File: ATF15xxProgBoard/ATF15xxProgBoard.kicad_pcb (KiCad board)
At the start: 4 copper layers, 71.1 x 96.2 mm, 42 parts, among them J1 Conn_02x05_Odd_Even, J10 Conn_02x03_Odd_Even, J2 Conn_02x07_Odd_Even, J6 Conn_02x16_Counter_Clockwise, J7 Conn_02x16_Counter_Clockwise, J8 Conn_02x03_Odd_Even, J9 USB_C, U3 ATmega32U4-AU, U4 MT3540, U5 AP2127K-3.3, Y1 8MHz

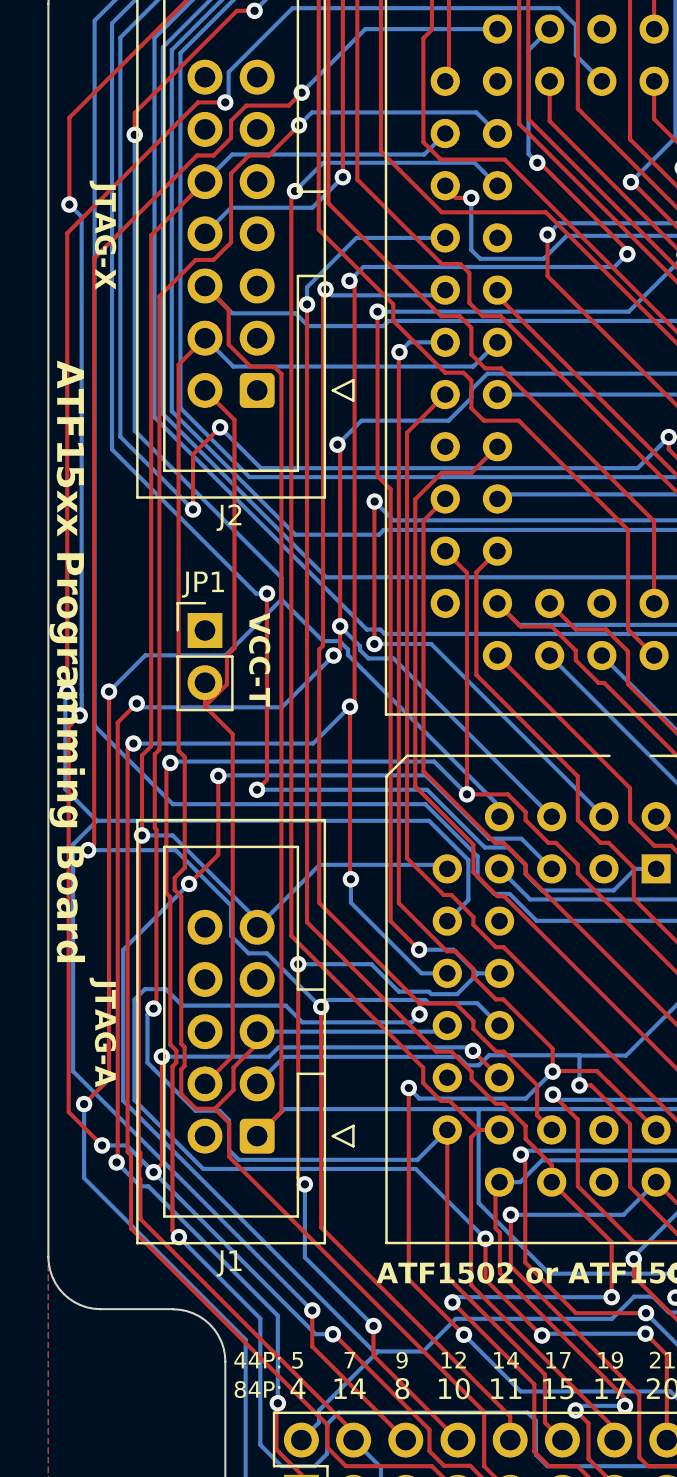
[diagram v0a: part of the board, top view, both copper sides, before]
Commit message: Open sourcing
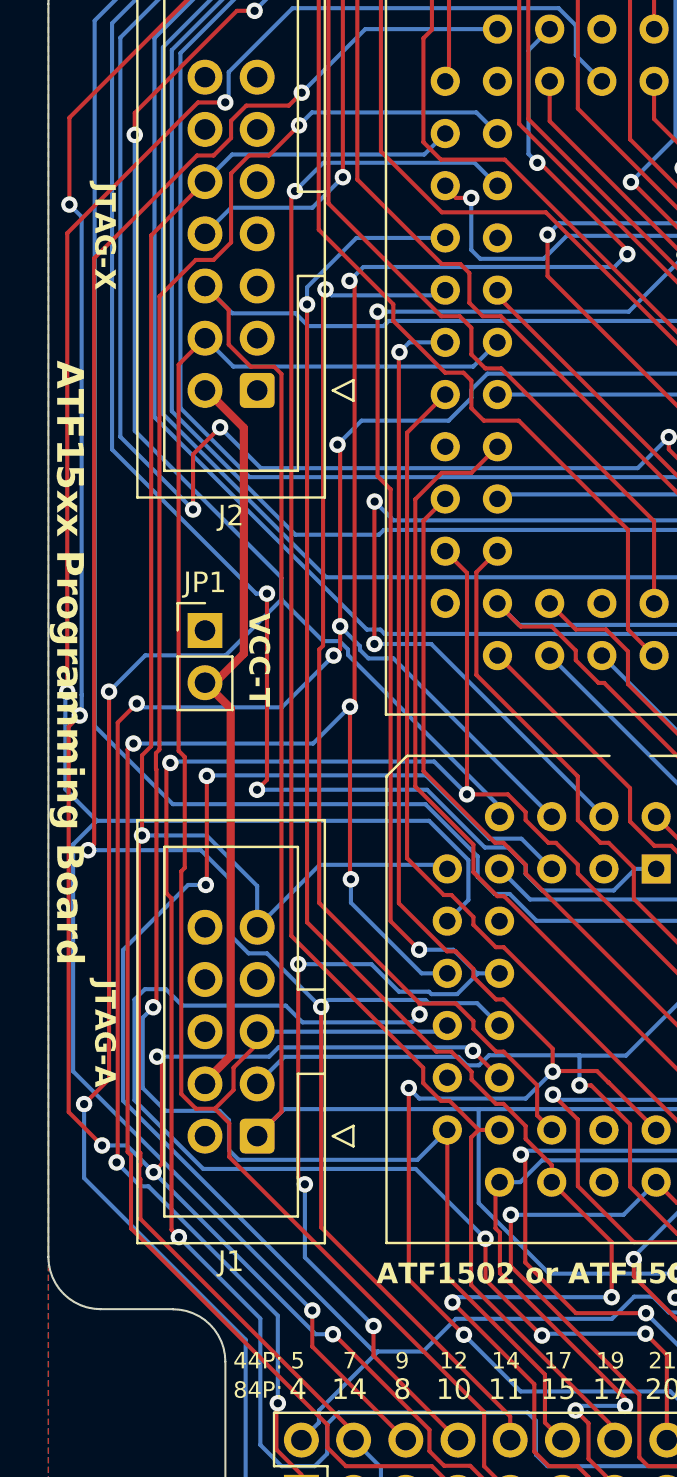
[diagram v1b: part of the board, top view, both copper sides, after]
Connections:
- JP1 pad 1: unconnected-(JP1-A-Pad1) -> VCC
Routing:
- net /IO12: track 95.5 -> 96.6 mm
- net TDI: track 158.3 -> 159.3 mm
- net /IO2: track 154.7 -> 155.5 mm
- net /IO10: track 103.2 -> 103.9 mm
- net Net-(J1-Pin_4): track 37.2 -> 36.7 mm
